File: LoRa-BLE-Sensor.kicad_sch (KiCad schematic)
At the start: 111 parts, among them J1 SHF-105-01-X-D-SM, J2 Battery_Cell, J3 Conn_01x06_Socket, J5 Screw_Terminal_01x06, J6 Screw_Terminal_01x06, J7 Conn_01x10_Pin, Q1 DMN67D7L, Q10 SQ2389ES, Q11 DMN62D0UDW-7, Q12 DMN62D0UDW-7, Q2 DMN67D7L, Q3 DMN67D7L, Q4 DMN67D7L, Q5 DMN67D7L, Q6 DMN67D7L, Q7 DMN67D7L, Q8 DMN67D7L, Q9 SQ2389ES, SW1 SW_Push, SW2 SW_Push, SW3 SW_Push, U1 RAK4630, U2 NPM1300-QEAA-R, U3 TLV61046ADBVR, U4 TLV61046ADBVR

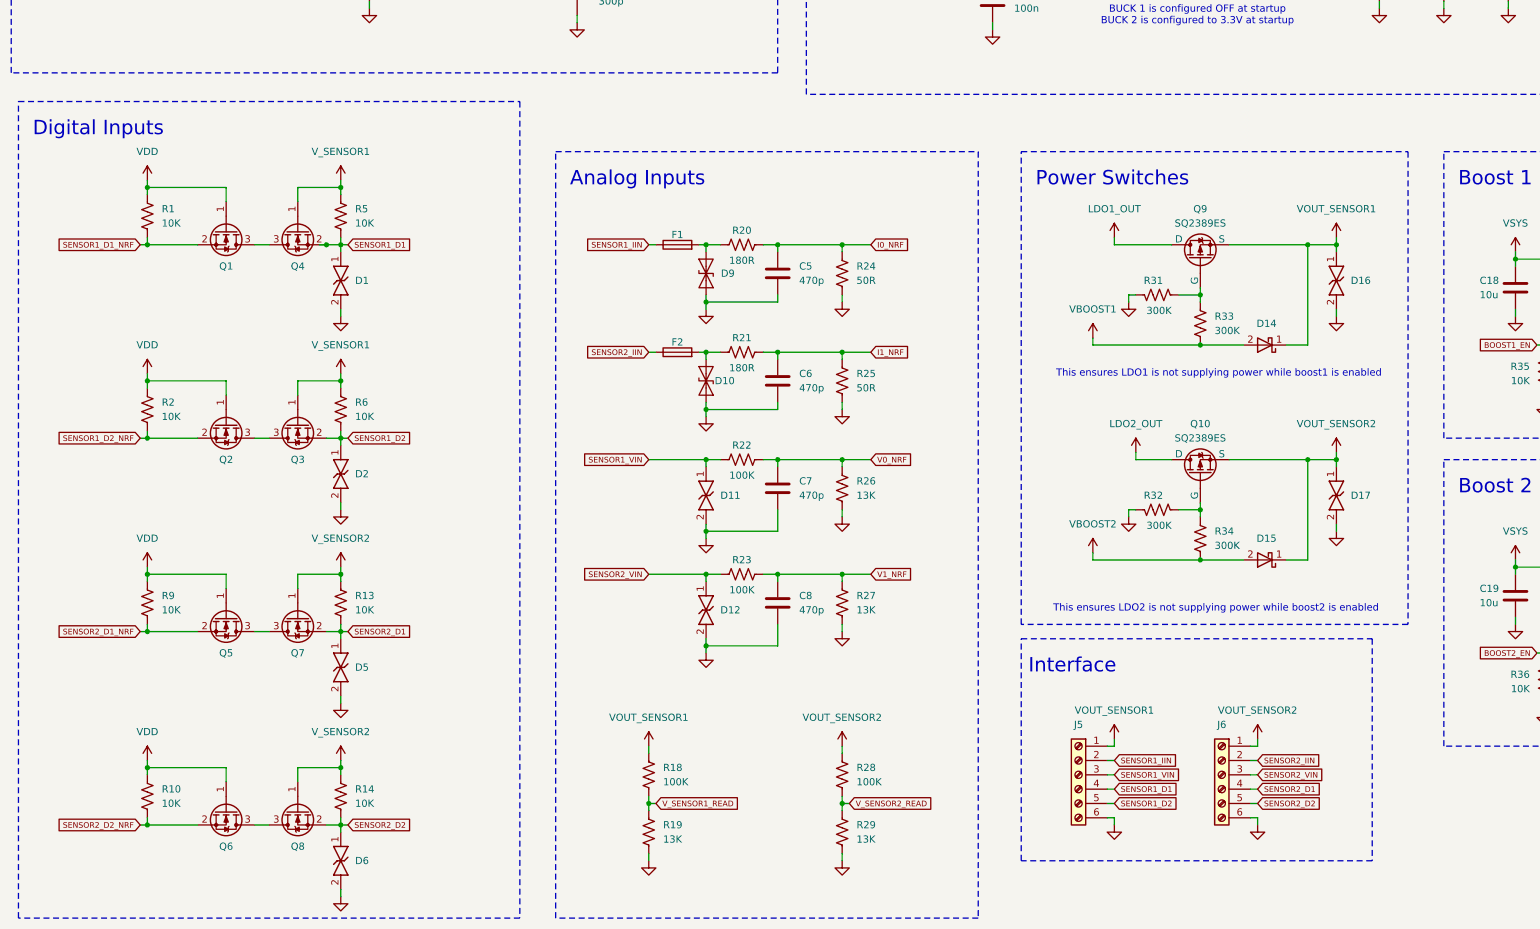
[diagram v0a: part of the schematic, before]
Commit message: update
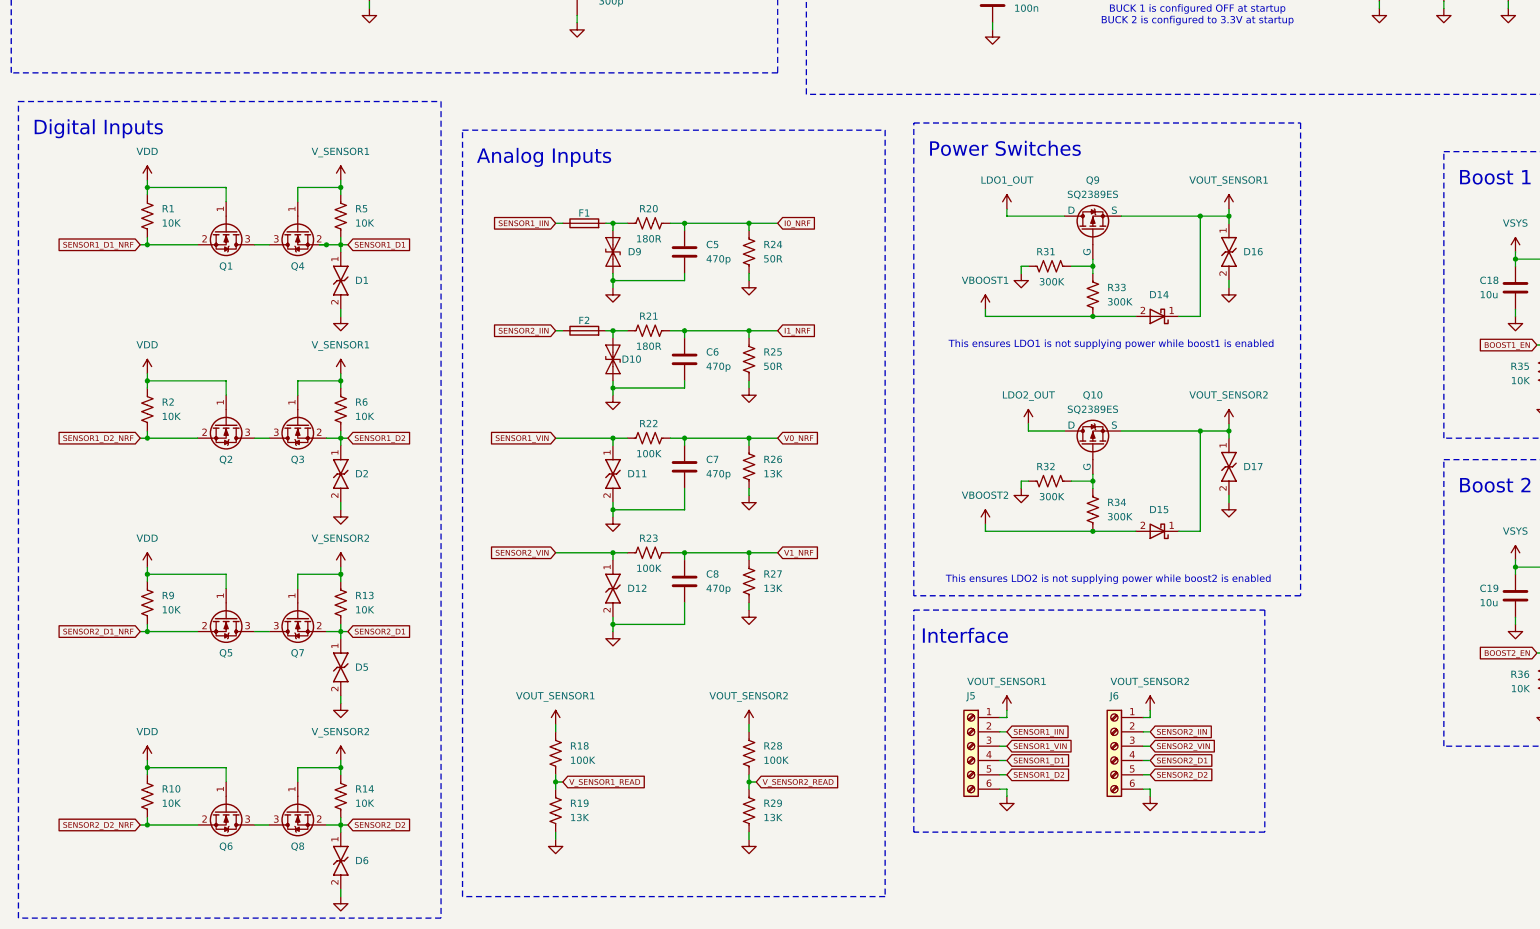
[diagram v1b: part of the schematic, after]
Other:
- moved on the sheet: C5, C6, C7, C8, D10, D11, D12, D14, D15, D16, D17, D9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
